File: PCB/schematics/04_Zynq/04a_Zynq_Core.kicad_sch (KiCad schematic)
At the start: 132 parts, among them U26 xczu4evfbvb900pkg

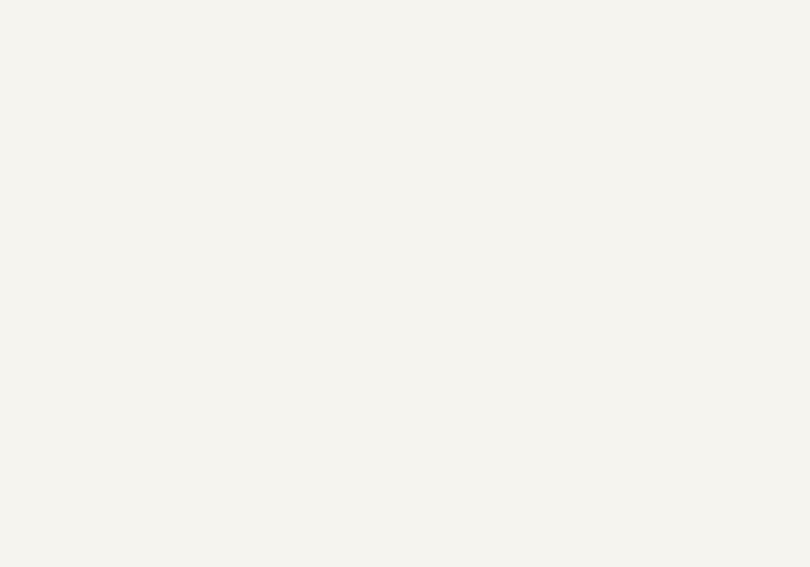
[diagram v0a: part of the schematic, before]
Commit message: Feat : Completed 04d Peripherals
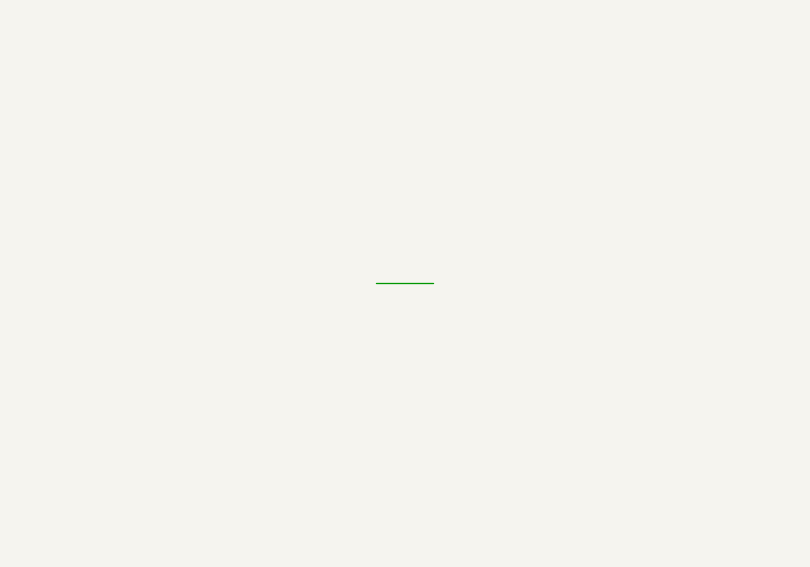
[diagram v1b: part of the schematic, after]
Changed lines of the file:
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@@
 	(generator "eeschema")
 	(generator_version "10.0")
-	(paper "User" 1300 1300)
+	(paper "User" 1300 1500)
 	(title_block
 		(date "2026-10-24")
@@
 		)
 		(stroke
+			(width 0)
+			(type default)
+		)
+	)
+	(wire
+		(pts
+			(xy 1008.38 582.93) (xy 1014.73 582.93)
+		)
+		(stroke

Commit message: Added 04D High Speed Peripherals
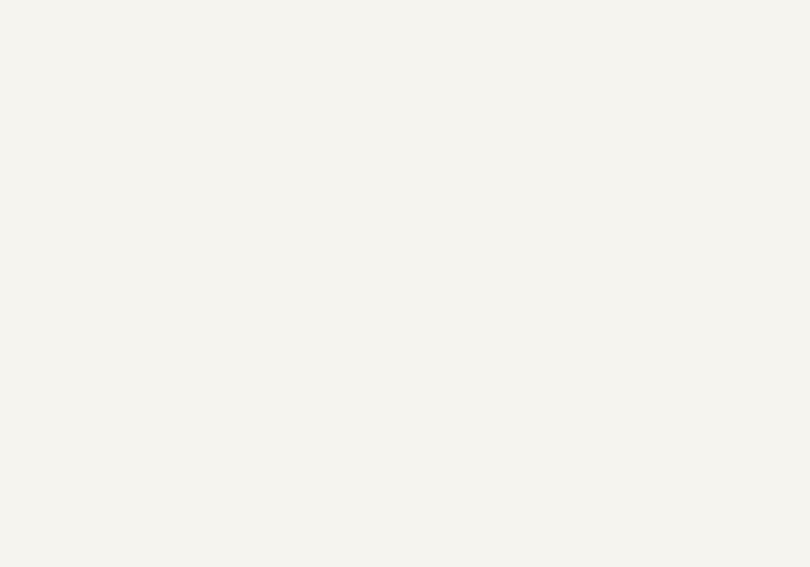
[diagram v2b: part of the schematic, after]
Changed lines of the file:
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@@
-	(wire
-		(pts
-			(xy 1008.38 582.93) (xy 1014.73 582.93)
-		)
-		(stroke
-			(width 0)
-			(type default)
-		)
-	)
 	(wire
 		(pts
